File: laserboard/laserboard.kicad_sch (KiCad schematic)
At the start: 0 parts

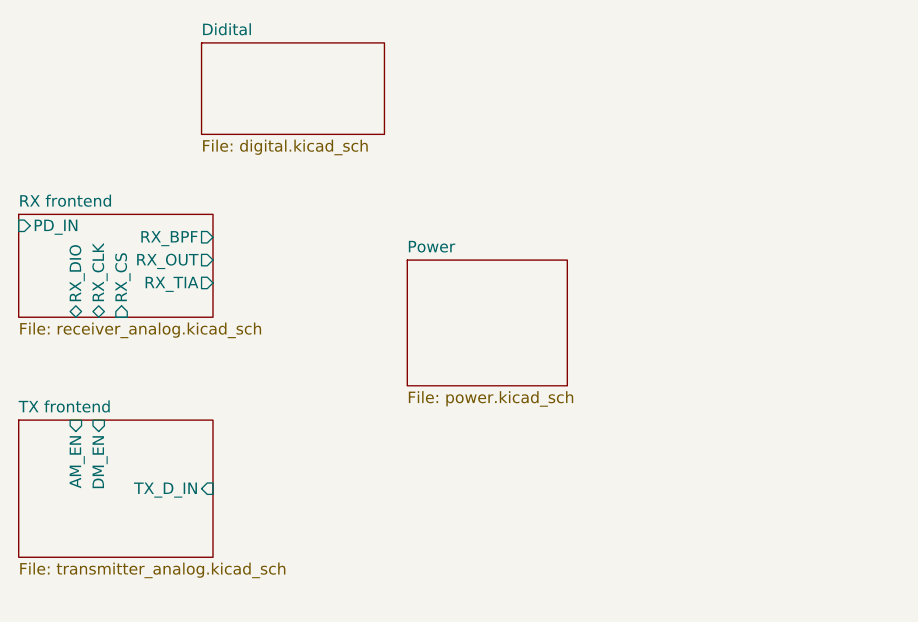
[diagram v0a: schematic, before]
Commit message: Pre-PCB backup
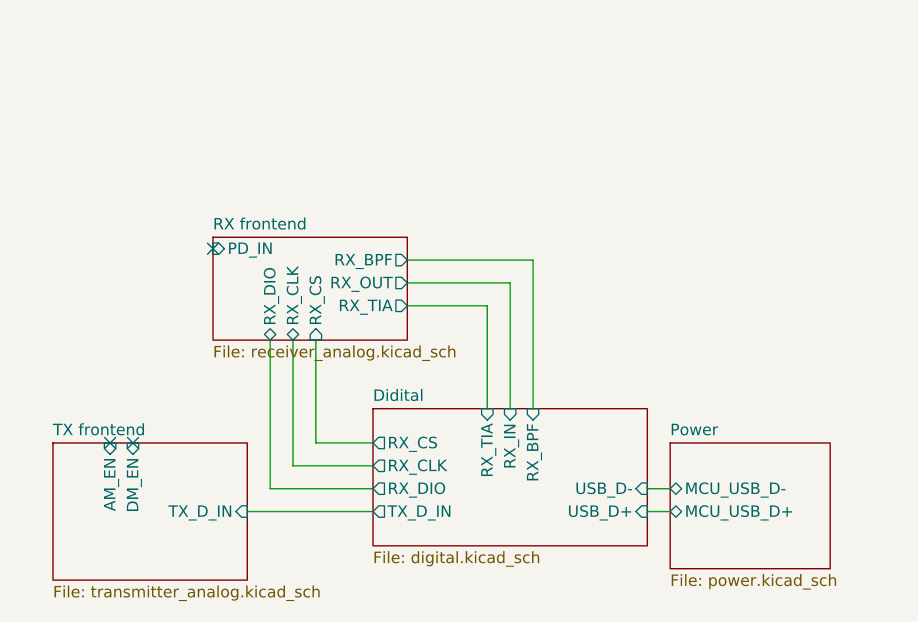
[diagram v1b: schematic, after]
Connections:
- no-connect marks 0 -> 3
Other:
- sheet Didital ports: added RX_BPF, RX_CLK, RX_CS, RX_DIO, RX_IN, RX_TIA, TX_D_IN, USB_D+, USB_D-; removed none
- sheet Power ports: added MCU_USB_D+, MCU_USB_D-; removed none
